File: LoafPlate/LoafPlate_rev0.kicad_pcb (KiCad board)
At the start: 2 copper layers, 195.1 x 84 mm, 1 part

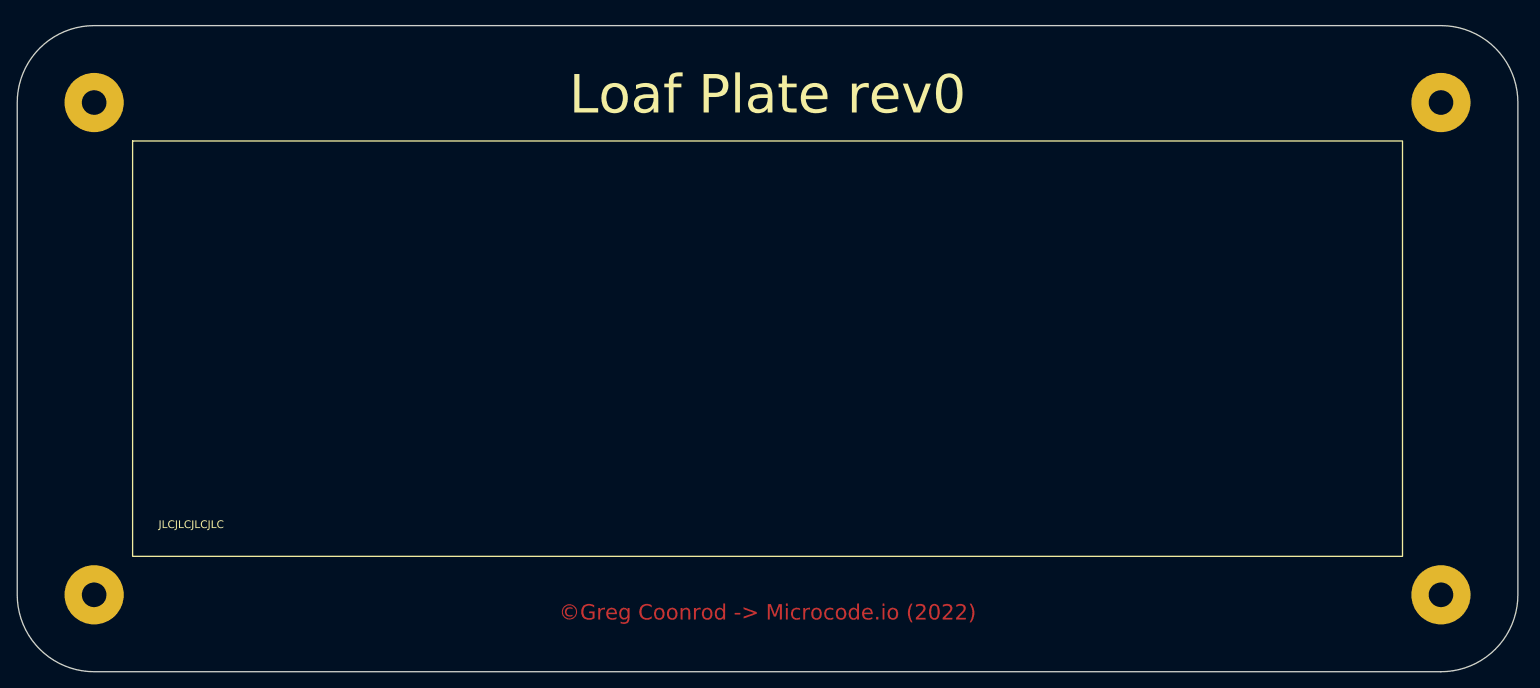
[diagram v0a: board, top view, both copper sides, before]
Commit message: Minor power revisions
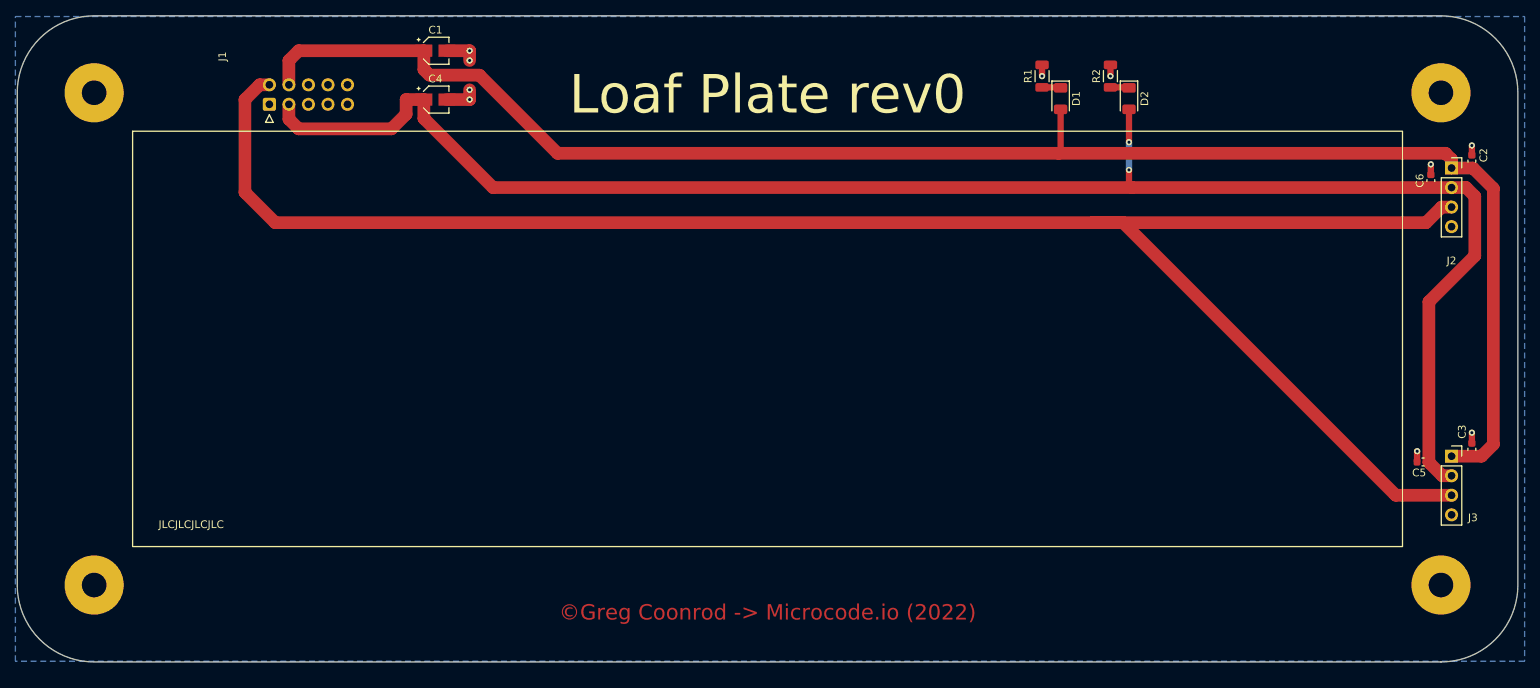
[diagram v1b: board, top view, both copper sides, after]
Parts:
- removed REF**: Breadboard_Bus_2_Terminal_1_Ties_830, CustomFootprintLibrary:Breadboard_Busx02_Terminalx01_Tiesx830_WithMounts
- added C1: 1p, Capacitor_SMD:CP_Elec_3x5.3, F.Cu at (106.7, 60.3)
- added C2: 100n, Capacitor_SMD:C_0603_1608Metric, F.Cu at (241.4, 74.7)
- added C3: 100n, Capacitor_SMD:C_0603_1608Metric, F.Cu at (241.4, 112.1)
- added C4: 1p, Capacitor_SMD:CP_Elec_3x5.3, F.Cu at (106.7, 66.7)
- added C5: 100n, Capacitor_SMD:C_0603_1608Metric, F.Cu at (235.1, 113.8)
- added C6: 100n, Capacitor_SMD:C_0603_1608Metric, F.Cu at (236.1, 77.2)
- added D1: +5V_PWR, LED_SMD:LED_1206_3216Metric, F.Cu at (188.0, 66.5)
- added D2: +3V3_PWR, LED_SMD:LED_1206_3216Metric, F.Cu at (196.8, 66.5)
- added J1: Ext Connector, Connector_IDC:IDC-Header_2x05_P2.54mm_Horizontal, F.Cu at (85.1, 67.3)
- added J2: Rail Power, Connector_PinSocket_2.54mm:PinSocket_1x04_P2.54mm_Vertical, F.Cu at (238.8, 75.6)
- added J3: Rail Power, Connector_PinSocket_2.54mm:PinSocket_1x04_P2.54mm_Vertical, F.Cu at (238.8, 113.0)
- added PLT1: BasePlate, CustomFootprintLibrary:Breadboard_Busx02_Terminalx01_Tiesx830_WithMounts, F.Cu at (149.9, 97.8)
- added R1: 120, Resistor_SMD:R_1206_3216Metric, F.Cu at (185.5, 63.6)
- added R2: 15, Resistor_SMD:R_1206_3216Metric, F.Cu at (194.4, 63.6)
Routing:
- net VCC: track 0.00 -> 236.7 mm
- net +3.3V: track 0.00 -> 217.0 mm, vias 0 -> 2
- net +5V: track 0.00 -> 215.0 mm
- net GND: track 0.00 -> 16.7 mm, vias 0 -> 10
- net Net-(D1-Pad1): track 0.00 -> 2.44 mm
- net Net-(D2-Pad1): track 0.00 -> 2.44 mm
- added copper zone on B.Cu, net GND
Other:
- rule pad_to_mask_clearance: 0 -> 0.05
